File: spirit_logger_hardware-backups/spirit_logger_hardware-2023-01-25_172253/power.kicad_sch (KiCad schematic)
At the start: 13 parts, among them U6 LMZ21700SILR, U7 SiP32432DR3

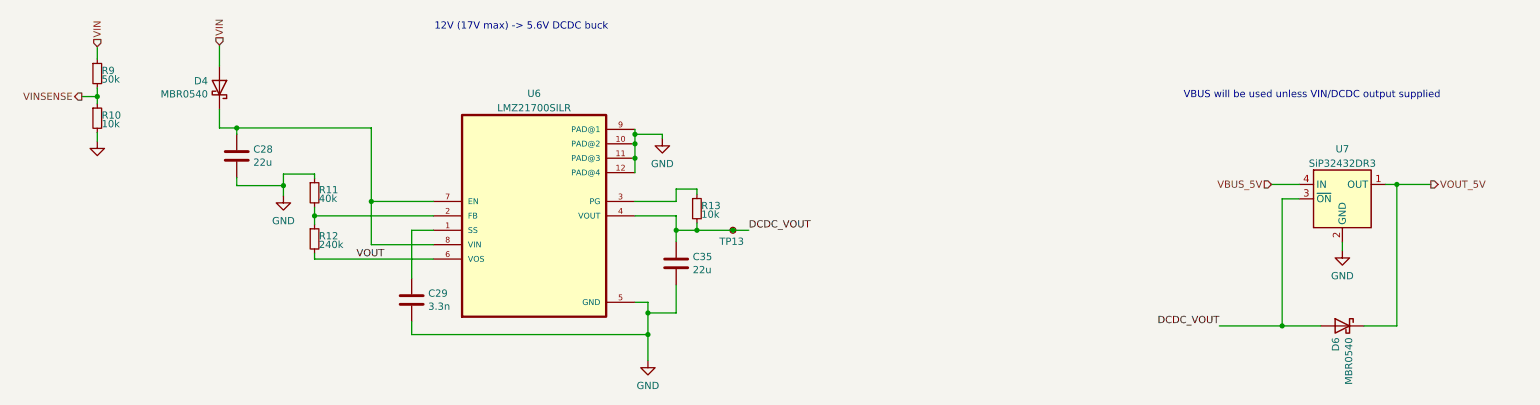
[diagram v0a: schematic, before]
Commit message: drc and packaging
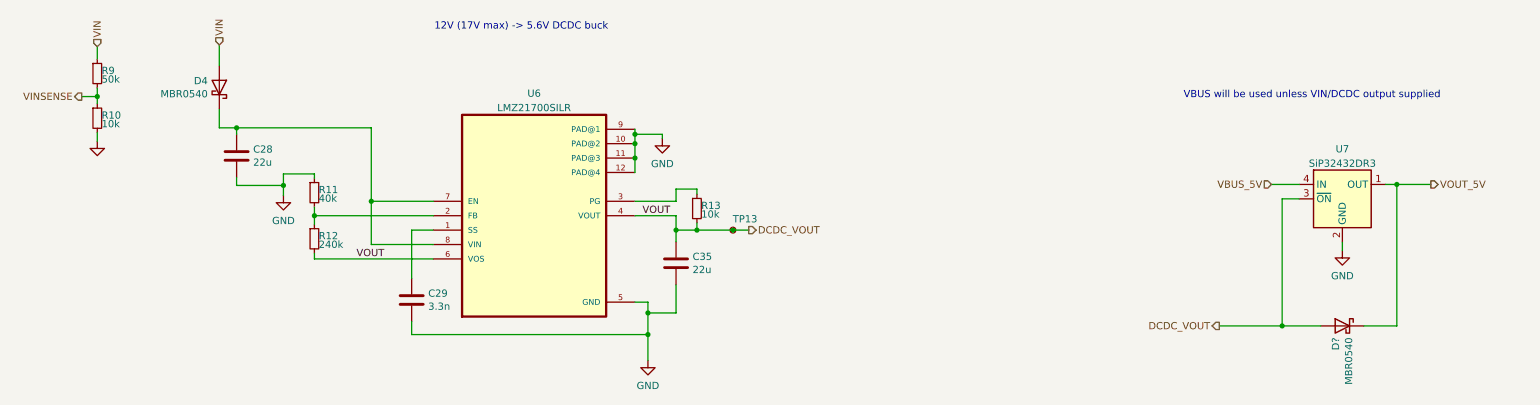
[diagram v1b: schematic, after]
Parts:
- C28, C35: footprint Capacitor_SMD:C_0805_2012Metric -> Capacitor_SMD.pretty:C_0805_2012Metric
- C29: footprint MCU_Nordic_Accessory:C_0201 -> Capacitor_SMD.pretty:C_0402_1005Metric
- D4: footprint Diode_SMD:D_SOD-123 -> Diode_SMD.pretty:D_SOD-123
- D?: renamed from D6; footprint Diode_SMD:D_SOD-123 -> Diode_SMD.pretty:D_SOD-123
- R10, R11, R12, R13, R9: footprint Resistor_SMD:R_0201_0603Metric -> Resistor_SMD.pretty:R_0402_1005Metric
- TP13: footprint tuna-f1sh/jbr-kicad/Misc.pretty:TestPoint_Pad_D1.0mm_Tight -> tunaf1sh/misc.pretty:TestPoint_Pad_D1.0mm_Tight
- U6: footprint tuna-f1sh/jbr-kicad/SnapEDA.pretty:CONV_TPS82140SILR -> tunaf1sh/snapeda.pretty:CONV_TPS82140SILR
- U7: footprint Package_TO_SOT_SMD:SOT-363_SC-70-6 -> Package_TO_SOT_SMD.pretty:SOT-363_SC-70-6
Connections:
- net VOUT is gone; now on net DCDC_VOUT: R12.2, U6.6 (VOS)
